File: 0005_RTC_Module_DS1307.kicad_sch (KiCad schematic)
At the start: 6 parts, among them U1 DS1307+, Y1 32.768Khz

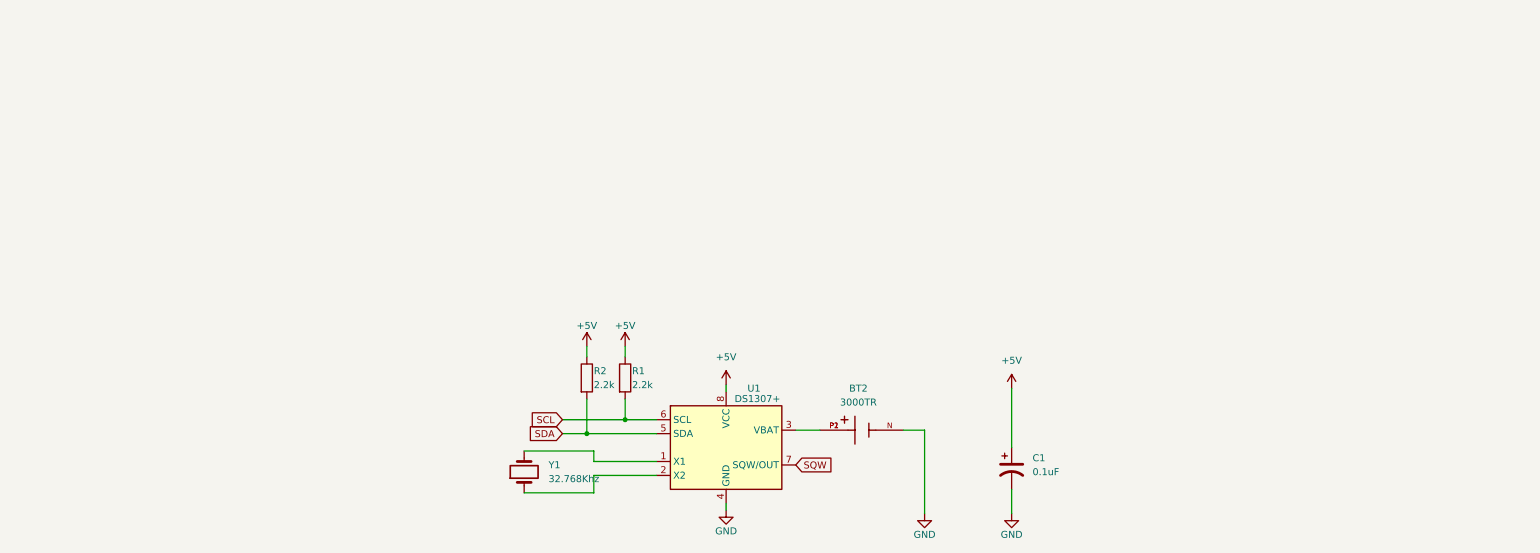
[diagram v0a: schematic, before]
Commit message: Add files via upload
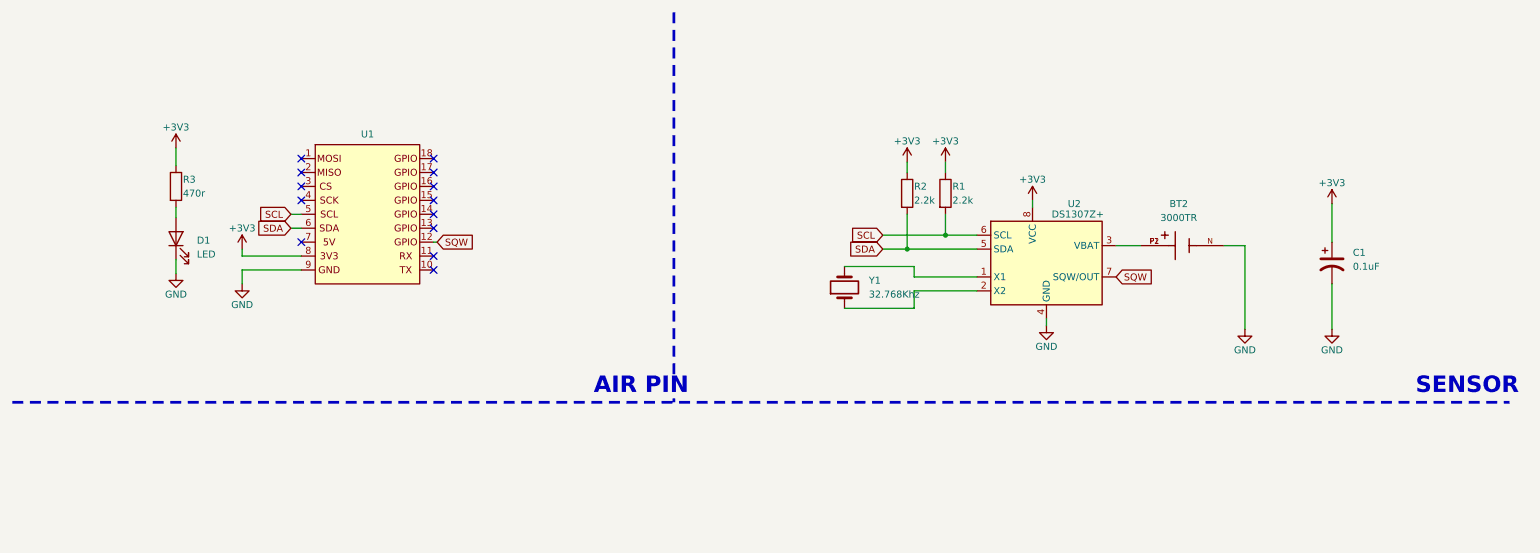
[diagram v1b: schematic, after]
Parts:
- removed U1: DS1307+, Package_DIP:DIP-8_W7.62mm, symbol Timer_RTC:DS1307+
- added D1: LED, LED_SMD:LED_0805_2012Metric, symbol Device:LED
- added R3: 470r, Resistor_SMD:R_0805_2012Metric, symbol Device:R
- added U1: ~, Moduler_:pin_header, symbol moduler_pin:air
- added U2: DS1307Z+, Package_SO:SOIC-8_3.9x4.9mm_P1.27mm, symbol Timer_RTC:DS1307Z+
- C1: footprint (none) -> Capacitor_SMD:T491A
- R1, R2: footprint (none) -> Resistor_SMD:R_0805_2012Metric
- Y1: footprint (none) -> Crystal:XTAL_ECS-.327-12.5-8X-C
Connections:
- net GND: now also D1.1 (K), U1.9, U2.4 (GND)
- net SCL: now also U1.5, U2.6 (SCL)
- net SDA: now also U1.6, U2.5 (SDA)
- net SQW: now also U1.12, U2.7 (SQW/OUT)
- net at Y1.1: now also U2.2 (X2)
- net at Y1.2: now also U2.1 (X1)
- net at BT2.P1, BT2.P2: now also U2.3 (VBAT)
- net +5V renamed +3V3
- net +3V3: now also R3.1, U1.8, U2.8 (VCC)
- new net: D1.2 (A), R3.2
- no-connect marks 0 -> 13
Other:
- note added: "AIR PIN"
- note added: "SENSOR"
- moved on the sheet: BT2, C1, R1, R2, Y1
